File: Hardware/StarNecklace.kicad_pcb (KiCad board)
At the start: 2 copper layers, 55.1 x 54.6 mm, 15 parts, among them J1 Conn_02x03_Odd_Even, SW1 SW_SPDT, U1 ATtiny13A

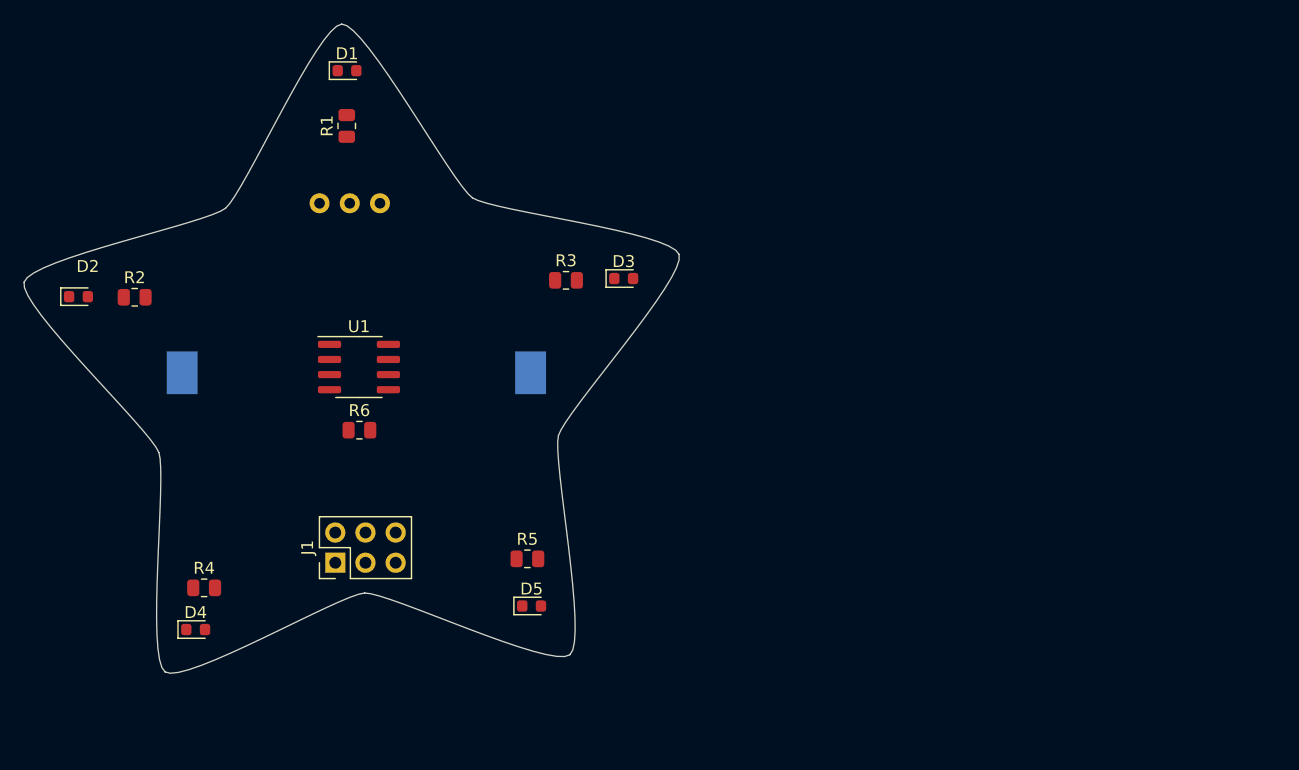
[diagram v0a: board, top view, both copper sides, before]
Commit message: feat: init routing
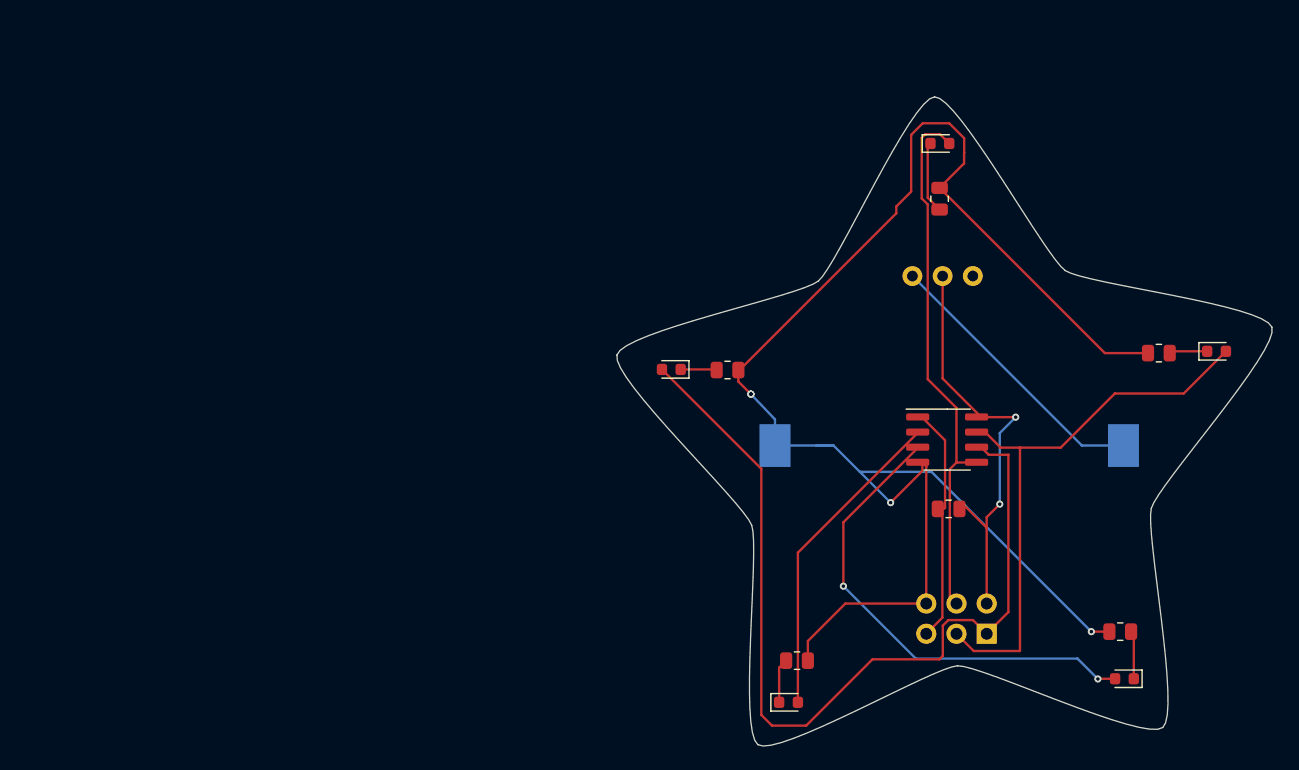
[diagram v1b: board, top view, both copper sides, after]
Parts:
- added G***: LOGO, LOGO, B.Cu at (97.8, 65.0)
- J1: moved to B.Cu
- moved J1 55.1 mm to (100.9, 80.8)
- moved D1 50.2 mm to (97.0, 39.6)
- moved D2 50.2 mm to (74.4, 58.6), turned to 180 degrees
- moved D4 50.2 mm to (84.2, 86.6)
- moved R1 50.2 mm to (96.9, 44.3)
- moved R2 50.2 mm to (79.1, 58.7)
- moved R3 50.2 mm to (115.4, 57.3), turned to 180 degrees
- moved BAT1 50.2 mm to (97.8, 65.0)
- moved D5 50.2 mm to (112.5, 84.6), turned to 180 degrees
- moved R4 50.2 mm to (85.0, 83.1)
- moved R5 50.2 mm to (112.1, 80.7), turned to 180 degrees
- moved SW1 50.2 mm to (97.2, 50.8)
- moved D3 50.2 mm to (120.2, 57.1)
- moved R6 50.0 mm to (97.7, 70.3), turned to 180 degrees
- moved U1 49.8 mm to (97.6, 64.5)
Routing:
- net GNDREF: track 0.00 -> 136.6 mm, vias 0 -> 4
- net MISO: track 0.00 -> 75.8 mm
- net SCK: track 0.00 -> 47.5 mm
- net MOSI: track 0.00 -> 45.7 mm
- net PB4: track 0.00 -> 40.8 mm, vias 0 -> 2
- net VCC: track 0.00 -> 35.6 mm, vias 0 -> 2
- net PB3: track 0.00 -> 27.2 mm
- net Net-(BAT1-+): track 0.00 -> 23.6 mm
- net RST: track 0.00 -> 20.7 mm
- net Net-(D1-K): track 0.00 -> 6.07 mm
- net Net-(D5-K): track 0.00 -> 4.06 mm
- net Net-(D4-K): track 0.00 -> 3.75 mm
- net Net-(D3-K): track 0.00 -> 3.21 mm
- net Net-(D2-K): track 0.00 -> 3.05 mm
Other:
- board text added: "Created by Angelina Tsuboi"
- board text added: "github.com/ANG13T/star_necklace_attiny13_smd"

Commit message: feat: init silk art
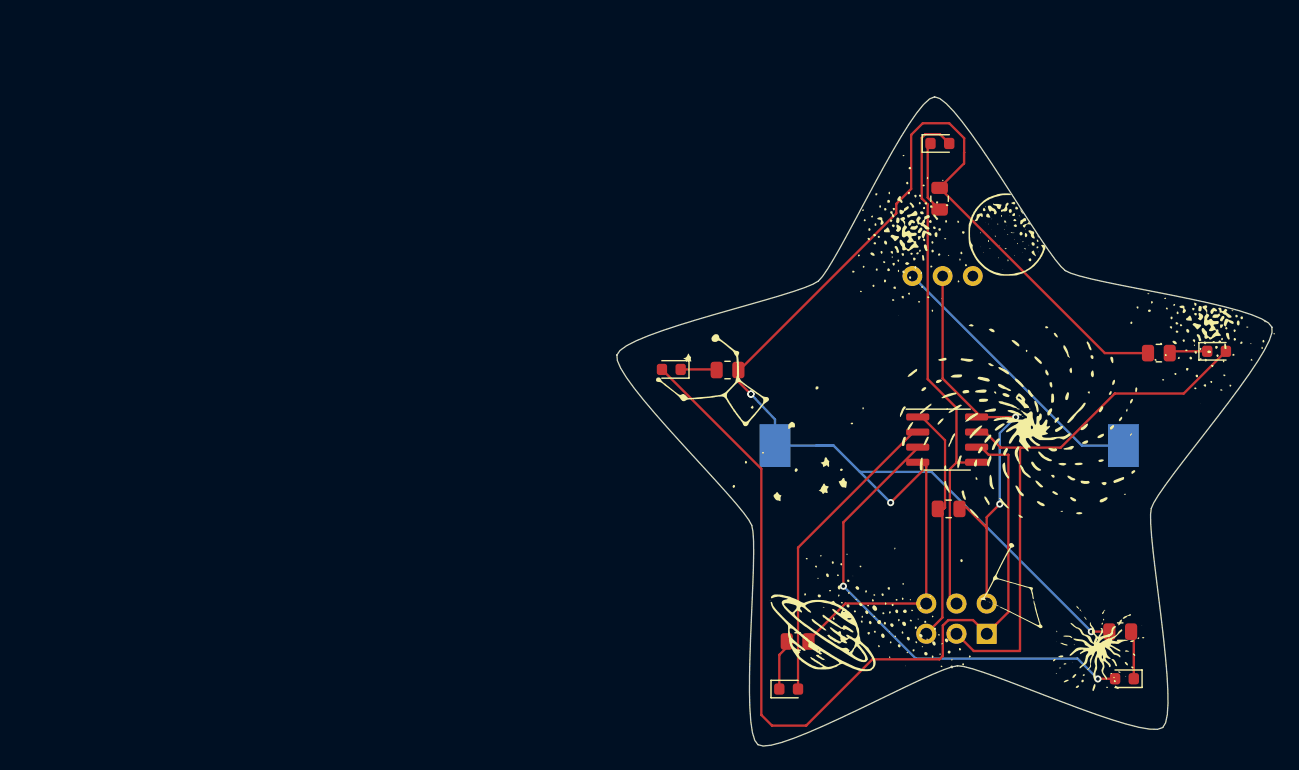
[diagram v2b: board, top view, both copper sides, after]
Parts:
- added G***: LOGO, LOGO, F.Cu at (98.8, 63.0)
- moved R4 1.61 mm to (85.0, 81.5)
- moved D4 1.12 mm to (84.2, 85.5)
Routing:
- net GNDREF: track 136.6 -> 135.0 mm
- net PB3: track 27.2 -> 26.1 mm
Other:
- board text added: "By Angelina Tsuboi"
- board text added: "angelinatsuboi.com"
- board text removed: "Created by Angelina Tsuboi"
- board text removed: "github.com/ANG13T/star_necklace_attiny13_smd"
